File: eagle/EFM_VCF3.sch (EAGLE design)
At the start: 33 parts, among them IC1 LM13700N, IC2 TL084P, Q3 2N3906, Q4 2N3906, U1 POWER

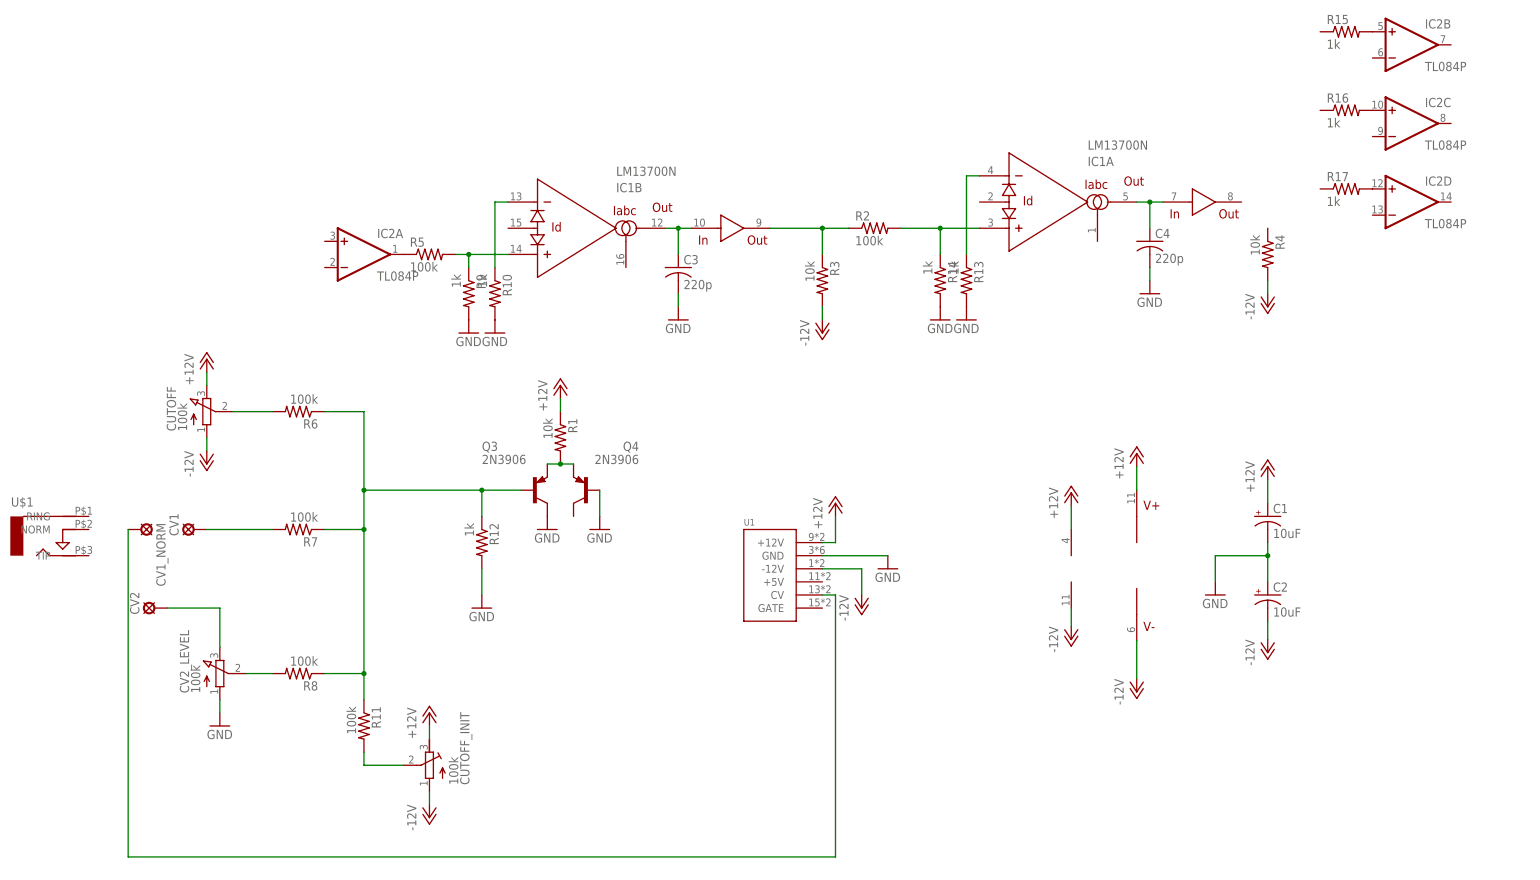
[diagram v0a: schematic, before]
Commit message: parts in place
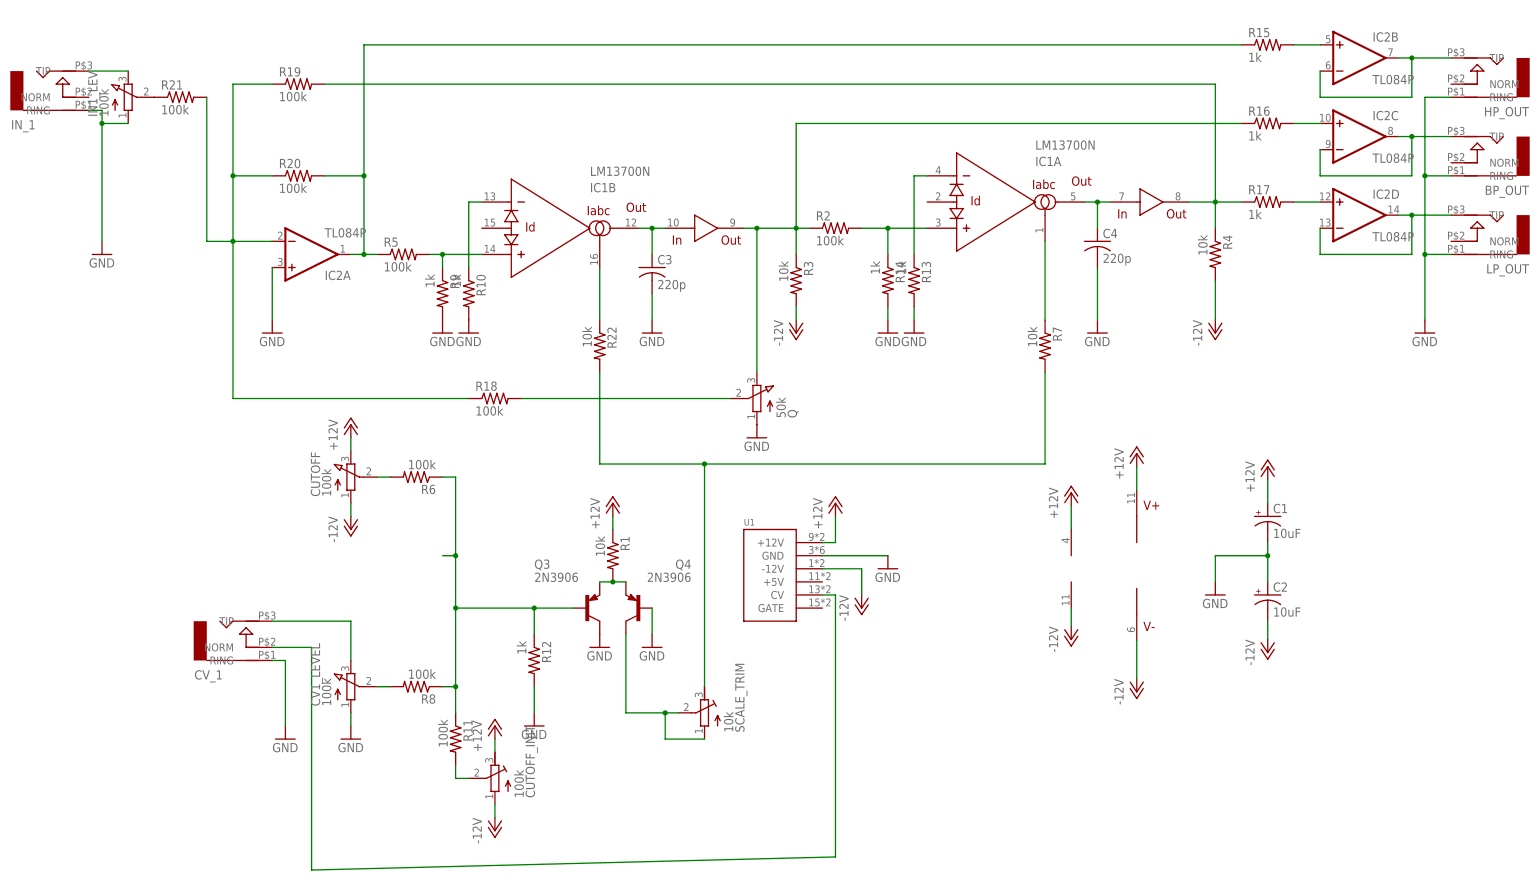
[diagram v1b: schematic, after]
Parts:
- removed CV1, CV1_NORM, CV2: LSP10, solpad:LSP10
- removed CV2_LEVEL: 100k, pot:3RP/1610N
- removed U$1: AUDIO-JACK, erthenvar:AUDIO-JACK
- added BP_OUT, CV_1, HP_OUT, IN_1, LP_OUT: AUDIO-JACK, erthenvar:AUDIO-JACK
- added CV1_LEVEL, IN1_LEV: 100k, pot:3RP/1610N
- added Q: 50k, pot:3RP/1610N
- added R18, R19, R20, R21: 100k, rcl:R-US_0207/7
- added R22: 10k, rcl:R-US_0207/7
- added SCALE_TRIM: 10k, rcl:R-TRIMM64W
- R7: value 100k -> 10k
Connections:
- removed net N$53: R7.2
- removed net N$59: CV1.MP
- new net N$14: IC2D.-IN, IC2D.OUT, LP_OUT.TIP
- new net N$15: BP_OUT.TIP, IC2C.-IN, IC2C.OUT
- new net N$17: HP_OUT.TIP, IC2B.-IN, IC2B.OUT
- new net N$18: Q3.B, R11.1, R12.1, R6.1, R8.1
- new net N$19: Q.S, R18.2
- new net N$20: IC1B.IABC, R22.1
- new net N$21: R22.2, R7.2, SCALE_TRIM.E
- new net N$22: IN1_LEV.E, IN_1.TIP
- new net N$23: IC1G$3.OUT, R17.1, R19.2, R4.1
- new net N$24: IN1_LEV.S, R21.1
- new net N$25: Q4.C, SCALE_TRIM.A, SCALE_TRIM.S
- new net N$26: IC2A.-IN, R18.1, R19.1, R20.1, R21.2
- net GND: now also BP_OUT.RING, CV1_LEVEL.A, CV_1.RING, HP_OUT.RING, IC2A.+IN, IN1_LEV.A, IN_1.RING, LP_OUT.RING, Q.A; no longer CV2_LEVEL.A
- net N$10: now also CV1_LEVEL.S; no longer CV2_LEVEL.S
- net N$16: now also IC1A.IABC; no longer Q3.B, R11.1, R12.1, R6.1, R8.1
- net N$5: now also Q.E, R16.1
- net N$54: now also CV1_LEVEL.E, CV_1.TIP; no longer CV2.MP, CV2_LEVEL.E
- net N$55: now also CV_1.NORM; no longer CV1_NORM.MP
- net N$9: now also R15.1, R20.2
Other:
- moved on the sheet: C3, C4, CUTOFF, CUTOFF_INIT, IC1A, IC1B, IC2A, IC2B, IC2C, IC2D, Q3, Q4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

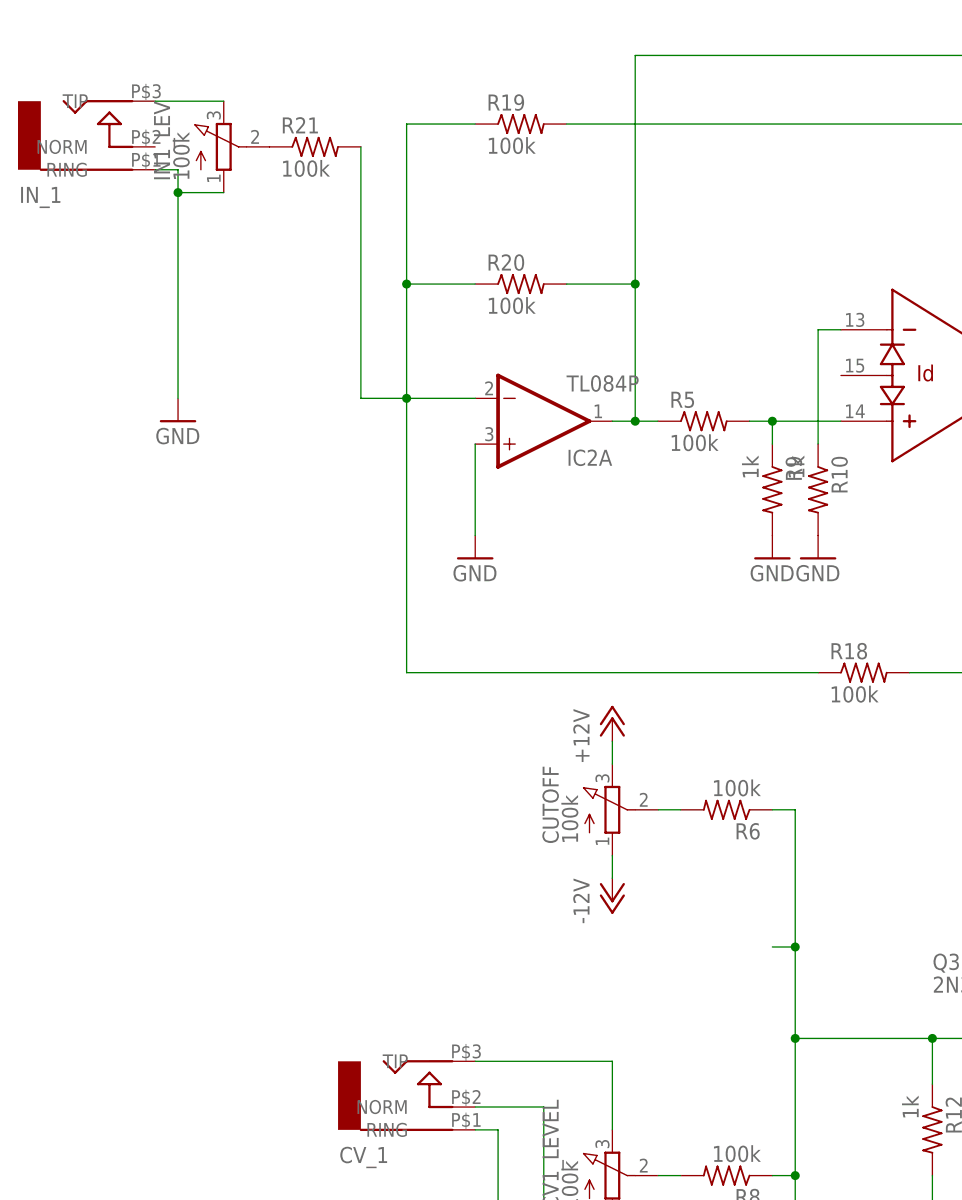
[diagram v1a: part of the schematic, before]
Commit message: started the board
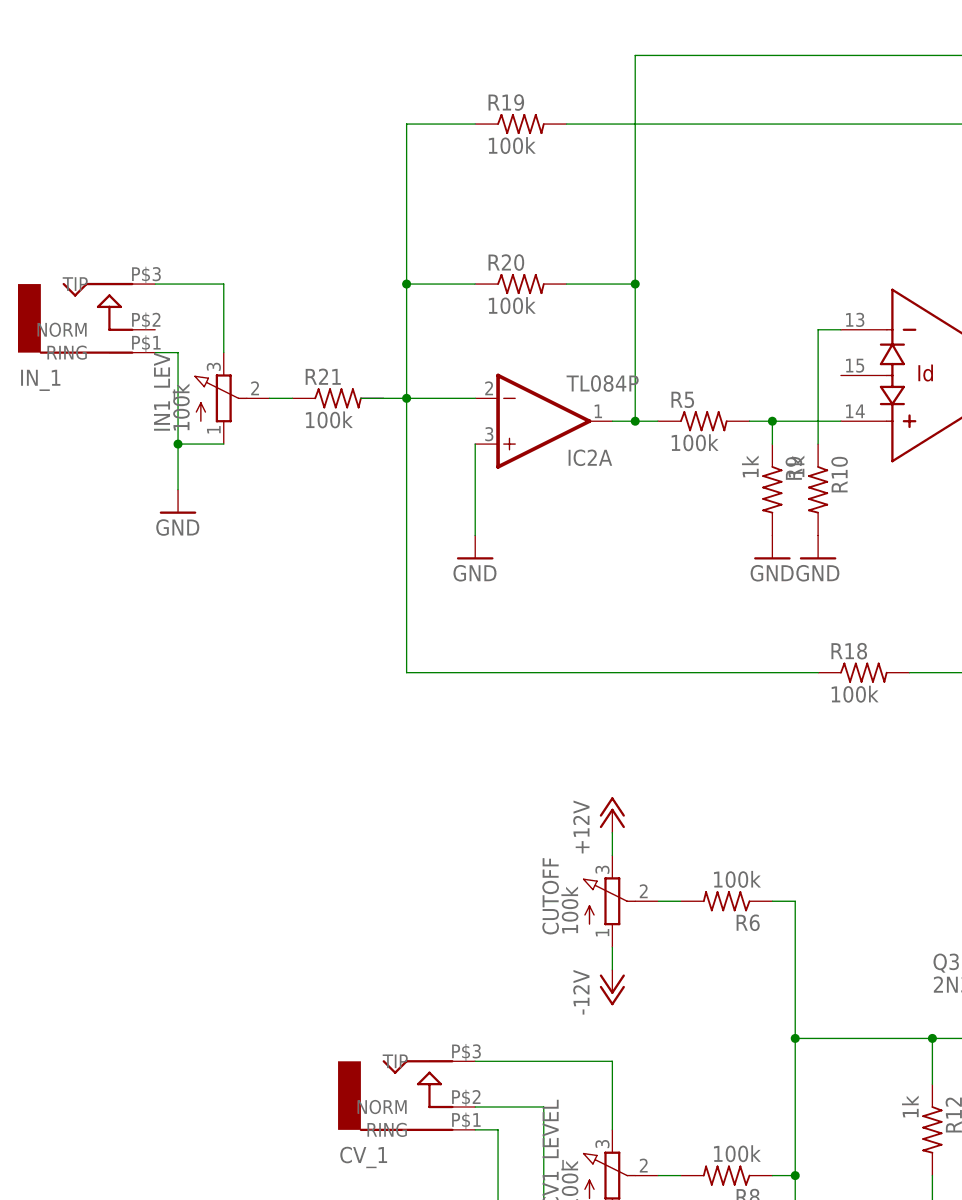
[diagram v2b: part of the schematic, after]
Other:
- moved on the sheet: CUTOFF, IN1_LEV, IN_1, R21, R6
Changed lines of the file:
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@@
 <instance part="P+4" gate="1" x="106.68" y="60.452"/>
 <instance part="P-3" gate="1" x="106.68" y="14.224"/>
-<instance part="CUTOFF" gate="G$1" x="-45.72" y="55.88"/>
-<instance part="P+3" gate="1" x="-45.72" y="66.04"/>
-<instance part="R6" gate="G$1" x="-33.02" y="55.88" rot="R180"/>
+<instance part="CUTOFF" gate="G$1" x="-45.72" y="45.72"/>
+<instance part="P+3" gate="1" x="-45.72" y="55.88"/>
+<instance part="R6" gate="G$1" x="-33.02" y="45.72" rot="R180"/>
 <instance part="P+1" gate="1" x="132.08" y="57.912"/>
 <instance part="P-1" gate="1" x="132.08" y="21.844"/>
@@
 <instance part="R16" gate="G$1" x="132.08" y="124.46"/>
 <instance part="R17" gate="G$1" x="132.08" y="109.22"/>
-<instance part="P-7" gate="1" x="-45.72" y="45.72"/>
+<instance part="P-7" gate="1" x="-45.72" y="35.56"/>
 <instance part="IC2" gate="A" x="-53.34" y="99.06" rot="MR180"/>
 <instance part="IC2" gate="B" x="149.86" y="137.16"/>
@@
 <instance part="R18" gate="G$1" x="-17.78" y="71.12"/>
 <instance part="GND16" gate="1" x="-60.96" y="83.82"/>
-<instance part="IN_1" gate="G$1" x="-104.14" y="129.54" rot="MR180"/>
-<instance part="GND17" gate="1" x="-93.98" y="99.06"/>
+<instance part="IN_1" gate="G$1" x="-104.14" y="109.22" rot="MR180"/>
+<instance part="GND17" gate="1" x="-93.98" y="88.9"/>
 <instance part="R19" gate="G$1" x="-55.88" y="132.08"/>
 <instance part="R20" gate="G$1" x="-55.88" y="114.3"/>
-<instance part="IN1_LEV" gate="G$1" x="-88.9" y="129.54"/>
-<instance part="R21" gate="G$1" x="-78.74" y="129.54"/>
+<instance part="IN1_LEV" gate="G$1" x="-88.9" y="101.6"/>
+<instance part="R21" gate="G$1" x="-76.2" y="101.6"/>
 <instance part="R7" gate="G$1" x="88.9" y="81.28" rot="R270"/>
 <instance part="R22" gate="G$1" x="2.54" y="81.28" rot="R270"/>
@@
 <pinref part="GND17" gate="1" pin="GND"/>
 <pinref part="IN_1" gate="G$1" pin="RING"/>
-<wire x1="-93.98" y1="101.6" x2="-93.98" y2="124.46" width="0.1524" layer="91"/>
-<wire x1="-93.98" y1="124.46" x2="-93.98" y2="127" width="0.1524" layer="91"/>
-<wire x1="-93.98" y1="127" x2="-96.52" y2="127" width="0.1524" layer="91"/>
+<wire x1="-93.98" y1="91.44" x2="-93.98" y2="96.52" width="0.1524" layer="91"/>
+<wire x1="-93.98" y1="96.52" x2="-93.98" y2="106.68" width="0.1524" layer="91"/>
+<wire x1="-93.98" y1="106.68" x2="-96.52" y2="106.68" width="0.1524" layer="91"/>
 <pinref part="IN1_LEV" gate="G$1" pin="A"/>
-<wire x1="-88.9" y1="124.46" x2="-93.98" y2="124.46" width="0.1524" layer="91"/>
-<junction x="-93.98" y="124.46"/>
+<wire x1="-88.9" y1="96.52" x2="-93.98" y2="96.52" width="0.1524" layer="91"/>
+<junction x="-93.98" y="96.52"/>
 </segment>
 </net>
@@
 <pinref part="CUTOFF" gate="G$1" pin="E"/>
 <pinref part="P+3" gate="1" pin="+12V"/>
-<wire x1="-45.72" y1="60.96" x2="-45.72" y2="63.5" width="0.1524" layer="91"/>
+<wire x1="-45.72" y1="50.8" x2="-45.72" y2="53.34" width="0.1524" layer="91"/>
 </segment>
 <segment>
@@
 <segment>
 <pinref part="CUTOFF" gate="G$1" pin="A"/>
-<wire x1="-45.72" y1="50.8" x2="-45.72" y2="48.26" width="0.1524" layer="91"/>
+<wire x1="-45.72" y1="40.64" x2="-45.72" y2="38.1" width="0.1524" layer="91"/>
 <pinref part="P-7" gate="1" pin="-12V"/>
 </segment>
@@
 <pinref part="CUTOFF" gate="G$1" pin="S"/>
 <pinref part="R6" gate="G$1" pin="2"/>
-<wire x1="-38.1" y1="55.88" x2="-40.64" y2="55.88" width="0.1524" layer="91"/>
+<wire x1="-38.1" y1="45.72" x2="-40.64" y2="45.72" width="0.1524" layer="91"/>
 </segment>
 </net>
@@
 <segment>
 <pinref part="R6" gate="G$1" pin="1"/>
-<wire x1="-27.94" y1="55.88" x2="-25.4" y2="55.88" width="0.1524" layer="91"/>
+<wire x1="-27.94" y1="45.72" x2="-25.4" y2="45.72" width="0.1524" layer="91"/>
 <pinref part="R8" gate="G$1" pin="1"/>
 <wire x1="-25.4" y1="30.48" x2="-25.4" y2="15.24" width="0.1524" layer="91"/>
@@
 <junction x="-10.16" y="30.48"/>
 <pinref part="Q3" gate="G$1" pin="B"/>
-<wire x1="-27.94" y1="40.64" x2="-25.4" y2="40.64" width="0.1524" layer="91"/>
-<wire x1="-25.4" y1="30.48" x2="-25.4" y2="40.64" width="0.1524" layer="91"/>
 <junction x="-25.4" y="30.48"/>
-<wire x1="-25.4" y1="55.88" x2="-25.4" y2="40.64" width="0.1524" layer="91"/>
-<junction x="-25.4" y="40.64"/>
+<wire x1="-25.4" y1="45.72" x2="-25.4" y2="30.48" width="0.1524" layer="91"/>
 </segment>
 </net>
@@
 <pinref part="R18" gate="G$1" pin="2"/>
 <wire x1="-12.7" y1="71.12" x2="27.94" y2="71.12" width="0.1524" layer="91"/>
-</segment>
-</net>
-<net name="N$22" class="0">
-<segment>
-<pinref part="IN_1" gate="G$1" pin="TIP"/>
-<wire x1="-96.52" y1="134.62" x2="-88.9" y2="134.62" width="0.1524" layer="91"/>
-<pinref part="IN1_LEV" gate="G$1" pin="E"/>
 </segment>
 </net>
@@
 <pinref part="IN1_LEV" gate="G$1" pin="S"/>
 <pinref part="R21" gate="G$1" pin="1"/>
+<wire x1="-83.82" y1="101.6" x2="-81.28" y2="101.6" width="0.1524" layer="91"/>
 </segment>
 </net>
@@
 <segment>
 <pinref part="R21" gate="G$1" pin="2"/>
-<wire x1="-73.66" y1="129.54" x2="-73.66" y2="101.6" width="0.1524" layer="91"/>
+<wire x1="-71.12" y1="101.6" x2="-73.66" y2="101.6" width="0.1524" layer="91"/>
 <pinref part="R18" gate="G$1" pin="1"/>
 <wire x1="-22.86" y1="71.12" x2="-68.58" y2="71.12" width="0.1524" layer="91"/>
@@
 <wire x1="-60.96" y1="114.3" x2="-68.58" y2="114.3" width="0.1524" layer="91"/>
 <junction x="-68.58" y="114.3"/>
-<wire x1="-73.66" y1="101.6" x2="-68.58" y2="101.6" width="0.1524" layer="91"/>
+<wire x1="-71.12" y1="101.6" x2="-68.58" y2="101.6" width="0.1524" layer="91"/>
 </segment>
 </net>
@@
 </segment>
 </net>
+<net name="N$22" class="0">
+<segment>
+<pinref part="IN_1" gate="G$1" pin="TIP"/>
+<wire x1="-96.52" y1="114.3" x2="-88.9" y2="114.3" width="0.1524" layer="91"/>
+<pinref part="IN1_LEV" gate="G$1" pin="E"/>
+<wire x1="-88.9" y1="114.3" x2="-88.9" y2="106.68" width="0.1524" layer="91"/>
+</segment>
+</net>
